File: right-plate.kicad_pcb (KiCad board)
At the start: 2 copper layers, 208.8 x 114.3 mm, 42 parts

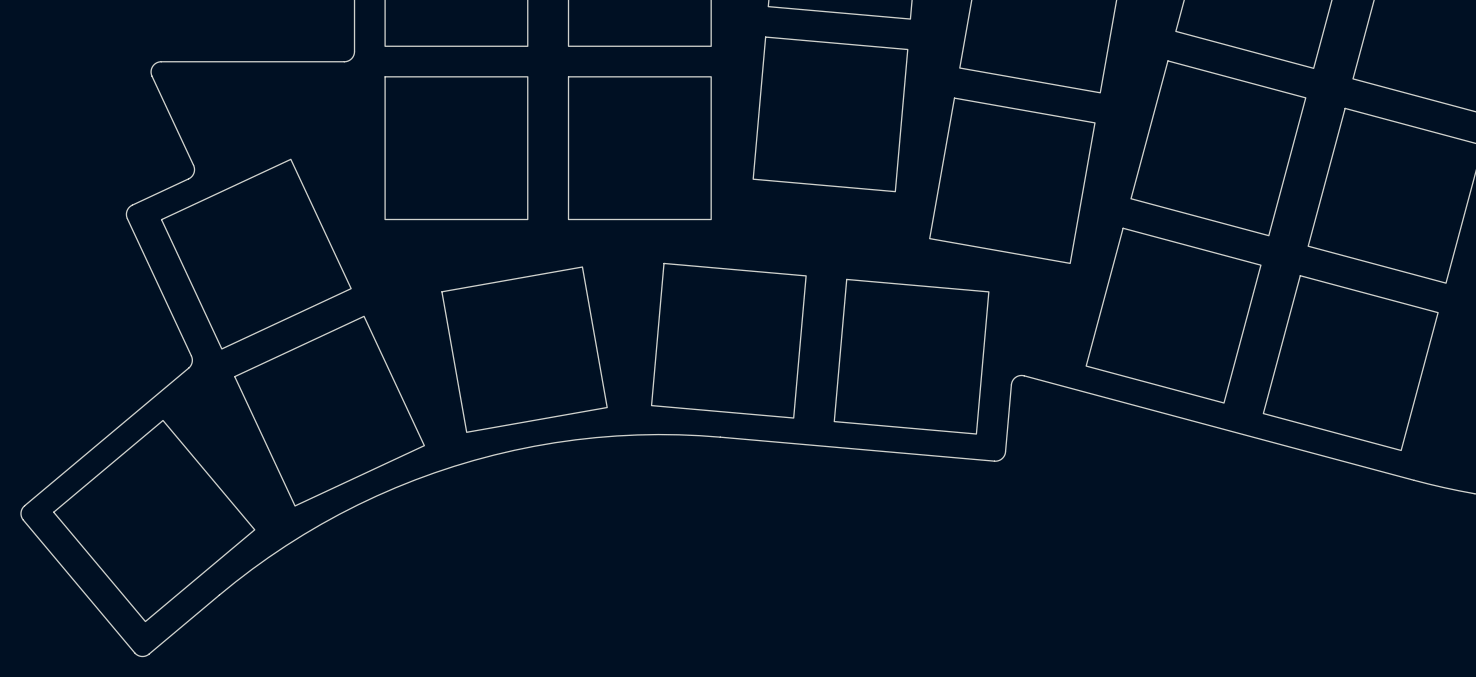
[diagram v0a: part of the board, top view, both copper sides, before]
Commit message: update plates
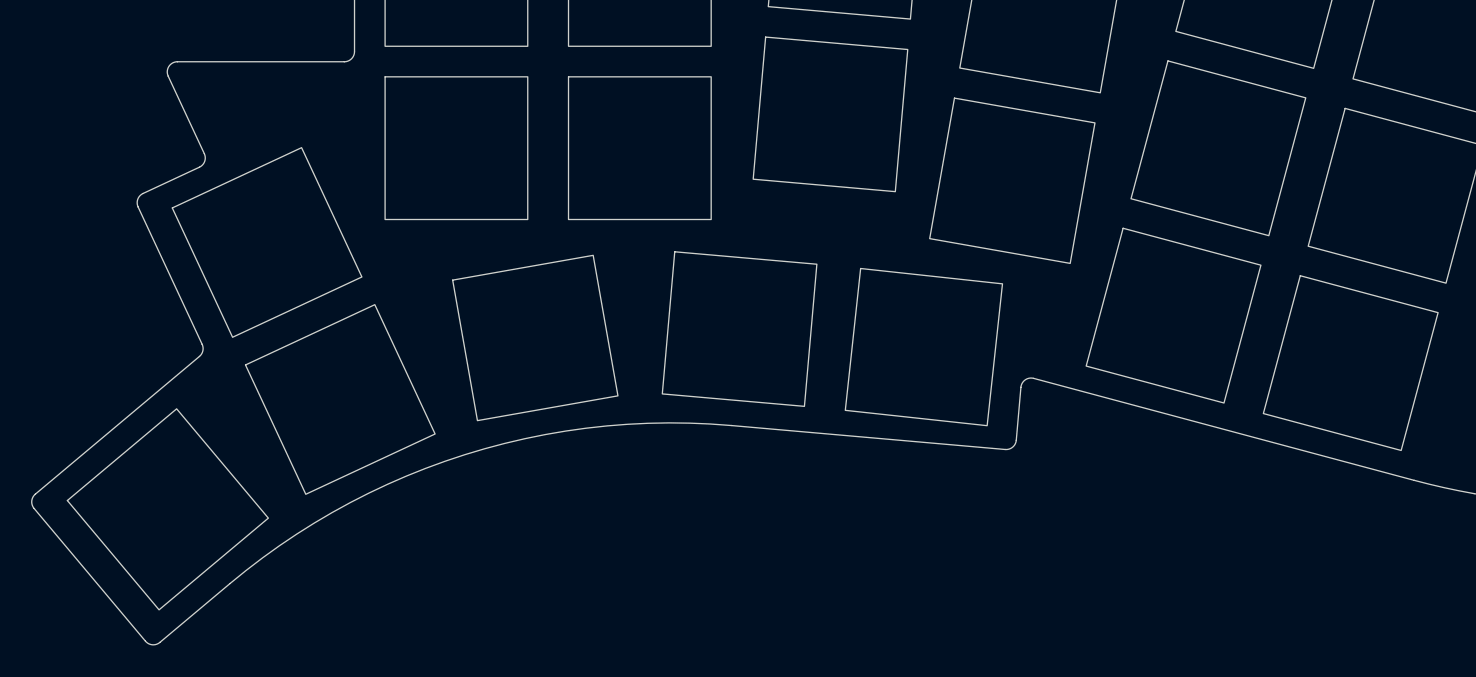
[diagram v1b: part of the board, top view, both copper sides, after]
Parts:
- moved REF** 1.76 mm to (51.5, 128.9)
- moved REF** 1.56 mm to (107.6, 111.3)
- moved REF** 1.56 mm to (68.4, 118.2)
- moved REF** 1.56 mm to (61.2, 102.8)
- moved REF** 1.56 mm to (87.5, 112.1)
- moved REF** 1.54 mm to (125.7, 113.0), turned to -6.171 degrees
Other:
- board size 208.8 x 114.3 mm -> 207.7 x 113.1 mm
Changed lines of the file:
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@@
   )
   (footprint "keyboard:KeyHole" (layer "F.Cu")
-    (at 60.145785 103.89932 25)
+    (at 61.201051 102.753693 25)
     (fp_text reference "REF**" (at 0 0 25 unlocked) (layer "F.Fab") hide
       (effects (font (size 1 1) (thickness 0.1)))
@@
   )
   (footprint "keyboard:KeyHole" (layer "F.Cu")
-    (at 106.512436 112.397684 -5)
+    (at 107.567703 111.252057 -5)
     (fp_text reference "REF**" (at 0 0 -5 unlocked) (layer "F.Fab") hide
       (effects (font (size 1 1) (thickness 0.1)))
@@
   )
   (footprint "keyboard:KeyHole" (layer "F.Cu")
-    (at 124.443941 113.966487 -5)
-    (fp_text reference "REF**" (at 0 0 -5 unlocked) (layer "F.Fab") hide
-      (effects (font (size 1 1) (thickness 0.1)))
-    )
-    (fp_text value "KeyHole" (at 0 2 -5 unlocked) (layer "F.Fab") hide
+    (at 125.654248 113.020897 -6.171)
+    (fp_text reference "REF**" (at 0 0 -6.171 unlocked) (layer "F.Fab") hide
+      (effects (font (size 1 1) (thickness 0.1)))
+    )
+    (fp_text value "KeyHole" (at 0 2 -6.171 unlocked) (layer "F.Fab") hide
       (effects (font (size 1 1) (thickness 0.125)))
     )
@@
   )
   (footprint "keyboard:KeyHole" (layer "F.Cu")
-    (at 67.330295 119.306552 25)
+    (at 68.385562 118.160925 25)
     (fp_text reference "REF**" (at 0 0 25 unlocked) (layer "F.Fab") hide
       (effects (font (size 1 1) (thickness 0.1)))
@@
   )
   (footprint "keyboard:KeyHole" (layer "F.Cu")
-    (at 86.466581 113.272904 10)
+    (at 87.521848 112.127278 10)
     (fp_text reference "REF**" (at 0 0 10 unlocked) (layer "F.Fab") hide
       (effects (font (size 1 1) (thickness 0.1)))
@@
   )
   (footprint "keyboard:KeyHole" (layer "F.Cu")
-    (at 50.124844 130.087443 40)
+    (at 51.462952 128.941816 40)
     (fp_text reference "REF**" (at 0 0 40 unlocked) (layer "F.Fab") hide
       (effects (font (size 1 1) (thickness 0.1)))
@@
     (fp_rect (start -7 -7) (end 7 7) (layer "Edge.Cuts") (stroke (width 0.12) (type default)) (fill none))
   )
-  (gr_line (start 49.909173 86.442618) (end 53.986308 95.186063) (layer "Edge.Cuts") (width 0.12))
-  (gr_line (start 47.490452 100.421886) (end 53.772947 113.894741) (layer "Edge.Cuts") (width 0.12))
+  (gr_line (start 51.498654 86.442618) (end 55.041575 94.040436) (layer "Edge.Cuts") (width 0.12))
+  (gr_line (start 48.545718 99.276259) (end 54.828214 112.749115) (layer "Edge.Cuts") (width 0.12))
   (gr_line (start 144.838586 37.117093) (end 153.701856 38.679926) (layer "Edge.Cuts") (width 0.12))
   (gr_line (start 179.650884 127.400816) (end 232.830502 136.777818) (layer "Edge.Cuts") (width 0.12))
   (gr_arc (start 244.985875 67.841276) (mid 245.631378 68.252507) (end 245.797034 68.999731) (layer "Edge.Cuts") (width 0.12))
   (gr_arc (start 111.710396 30.037309) (mid 112.063803 29.35842) (end 112.793746 29.12827) (layer "Edge.Cuts") (width 0.12))
-  (gr_arc (start 134.24122 116.720205) (mid 134.663841 115.988213) (end 135.496234 115.841441) (layer "Edge.Cuts") (width 0.12))
   (gr_arc (start 191.892252 58.479437) (mid 191.849455 58.470924) (end 191.80707 58.460552) (layer "Edge.Cuts") (width 0.12))
   (gr_line (start 70.78 33) (end 97.78 33) (layer "Edge.Cuts") (width 0.12))
@@
   (gr_arc (start 153.945198 48.315494) (mid 153.360626 47.886868) (end 153.219209 47.17592) (layer "Edge.Cuts") (width 0.12))
   (gr_arc (start 153.701856 38.679926) (mid 154.34736 39.091158) (end 154.513015 39.838382) (layer "Edge.Cuts") (width 0.12))
-  (gr_arc (start 53.772946 113.894741) (mid 53.842935 114.533799) (end 53.509427 115.083404) (layer "Edge.Cuts") (width 0.12))
-  (gr_line (start 53.509427 115.083404) (end 37.406804 128.59511) (layer "Edge.Cuts") (width 0.12))
+  (gr_line (start 54.564694 113.937777) (end 38.462071 127.449483) (layer "Edge.Cuts") (width 0.12))
+  (gr_arc (start 57.569435 136.219239) (mid 80.612677 123.577284) (end 106.739723 120.715907) (layer "Edge.Cuts") (width 0.12))
   (gr_line (start 131.42888 34.128269) (end 131.63429 31.780424) (layer "Edge.Cuts") (width 0.12))
-  (gr_line (start 68.78 85.02) (end 50.815481 85.02) (layer "Edge.Cuts") (width 0.12))
+  (gr_line (start 68.78 85.02) (end 52.404962 85.02) (layer "Edge.Cuts") (width 0.12))
   (gr_line (start 191.80707 58.460552) (end 153.945198 48.315494) (layer "Edge.Cuts") (width 0.12))
-  (gr_line (start 134.24122 116.720205) (end 133.665064 123.305699) (layer "Edge.Cuts") (width 0.12))
+  (gr_arc (start 50.675034 142.004326) (mid 49.945092 142.234476) (end 49.266203 141.88107) (layer "Edge.Cuts") (width 0.12))
+  (gr_arc (start 54.828214 112.749115) (mid 54.898202 113.388172) (end 54.564694 113.937777) (layer "Edge.Cuts") (width 0.12))
+  (gr_arc (start 48.545718 99.276259) (mid 48.512334 98.511621) (end 49.029408 97.947333) (layer "Edge.Cuts") (width 0.12))
+  (gr_line (start 135.17438 116.970262) (end 134.720331 122.160072) (layer "Edge.Cuts") (width 0.12))
   (gr_arc (start 233.988959 135.966658) (mid 233.577727 136.612162) (end 232.830502 136.777818) (layer "Edge.Cuts") (width 0.12))
   (gr_arc (start 97.78 33) (mid 104.122734 33.074236) (end 110.461994 33.296903) (layer "Edge.Cuts") (width 0.12))
-  (gr_line (start 53.502619 96.514989) (end 47.974141 99.09296) (layer "Edge.Cuts") (width 0.12))
-  (gr_line (start 173.774094 126.097962) (end 135.496234 115.841441) (layer "Edge.Cuts") (width 0.12))
+  (gr_line (start 54.557885 95.369362) (end 49.029408 97.947333) (layer "Edge.Cuts") (width 0.12))
+  (gr_line (start 173.774094 126.097962) (end 136.429395 116.091481) (layer "Edge.Cuts") (width 0.12))
+  (gr_arc (start 134.720331 122.160072) (mid 134.366924 122.838961) (end 133.63698 123.069112) (layer "Edge.Cuts") (width 0.12))
   (gr_arc (start 130.725251 30.697074) (mid 131.40414 31.050481) (end 131.63429 31.780424) (layer "Edge.Cuts") (width 0.12))
-  (gr_line (start 132.581714 124.214738) (end 105.684457 121.861533) (layer "Edge.Cuts") (width 0.12))
+  (gr_line (start 133.63698 123.069111) (end 106.739723 120.715906) (layer "Edge.Cuts") (width 0.12))
   (gr_line (start 111.710396 30.037309) (end 111.504986 32.385154) (layer "Edge.Cuts") (width 0.12))
+  (gr_arc (start 38.338814 128.858315) (mid 38.108663 128.128371) (end 38.462071 127.449482) (layer "Edge.Cuts") (width 0.12))
   (gr_arc (start 111.504986 32.385154) (mid 111.16694 33.050886) (end 110.461994 33.296902) (layer "Edge.Cuts") (width 0.12))
-  (gr_arc (start 47.490452 100.421886) (mid 47.457067 99.657248) (end 47.974141 99.09296) (layer "Edge.Cuts") (width 0.12))
   (gr_line (start 69.78 84.02) (end 69.78 34) (layer "Edge.Cuts") (width 0.12))
-  (gr_line (start 49.619768 143.149954) (end 56.514168 137.364866) (layer "Edge.Cuts") (width 0.12))
+  (gr_line (start 50.675034 142.004326) (end 57.569435 136.219239) (layer "Edge.Cuts") (width 0.12))
+  (gr_arc (start 51.498654 86.442618) (mid 51.56157 85.4827) (end 52.404962 85.02) (layer "Edge.Cuts") (width 0.12))
   (gr_line (start 191.892252 58.479437) (end 244.985875 67.841276) (layer "Edge.Cuts") (width 0.12))
   (gr_arc (start 69.78 84.02) (mid 69.487107 84.727107) (end 68.78 85.02) (layer "Edge.Cuts") (width 0.12))
   (gr_arc (start 69.78 34) (mid 70.072893 33.292893) (end 70.78 33) (layer "Edge.Cuts") (width 0.12))
   (gr_arc (start 132.2977 35.20728) (mid 138.579319 36.088797) (end 144.838586 37.117094) (layer "Edge.Cuts") (width 0.12))
-  (gr_line (start 48.210936 143.026697) (end 37.283547 130.003942) (layer "Edge.Cuts") (width 0.12))
+  (gr_line (start 49.266202 141.88107) (end 38.338813 128.858315) (layer "Edge.Cuts") (width 0.12))
   (gr_arc (start 179.650884 127.400815) (mid 176.698275 126.813504) (end 173.774094 126.097962) (layer "Edge.Cuts") (width 0.12))
-  (gr_arc (start 133.665064 123.305699) (mid 133.311657 123.984588) (end 132.581714 124.214738) (layer "Edge.Cuts") (width 0.12))
   (gr_line (start 154.513015 39.838382) (end 153.219209 47.17592) (layer "Edge.Cuts") (width 0.12))
-  (gr_arc (start 53.986308 95.186063) (mid 54.019693 95.950701) (end 53.502619 96.514988) (layer "Edge.Cuts") (width 0.12))
-  (gr_arc (start 49.909173 86.442618) (mid 49.97209 85.4827) (end 50.815481 85.02) (layer "Edge.Cuts") (width 0.12))
-  (gr_arc (start 49.619768 143.149954) (mid 48.889825 143.380104) (end 48.210937 143.026696) (layer "Edge.Cuts") (width 0.12))
+  (gr_arc (start 135.17438 116.970262) (mid 135.596995 116.238258) (end 136.429395 116.091481) (layer "Edge.Cuts") (width 0.12))
+  (gr_arc (start 55.041575 94.040436) (mid 55.074959 94.805074) (end 54.557885 95.369362) (layer "Edge.Cuts") (width 0.12))
   (gr_line (start 130.725251 30.697074) (end 112.793746 29.12827) (layer "Edge.Cuts") (width 0.12))
   (gr_line (start 233.988959 135.966658) (end 245.797034 68.999731) (layer "Edge.Cuts") (width 0.12))
-  (gr_arc (start 56.514168 137.364866) (mid 79.55741 124.72291) (end 105.684457 121.861534) (layer "Edge.Cuts") (width 0.12))
-  (gr_arc (start 37.283548 130.003941) (mid 37.053398 129.273999) (end 37.406804 128.59511) (layer "Edge.Cuts") (width 0.12))
 )
